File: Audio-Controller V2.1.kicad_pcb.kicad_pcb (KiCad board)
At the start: 2 copper layers, 73 x 100 mm, 12 parts

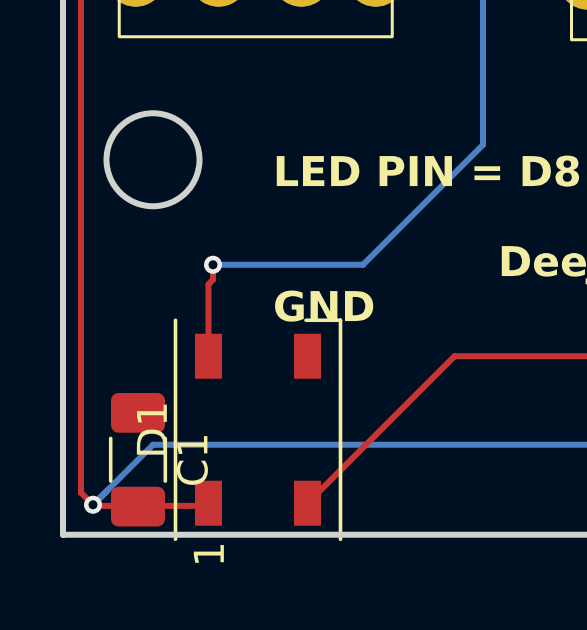
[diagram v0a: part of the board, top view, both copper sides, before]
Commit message: small corrections
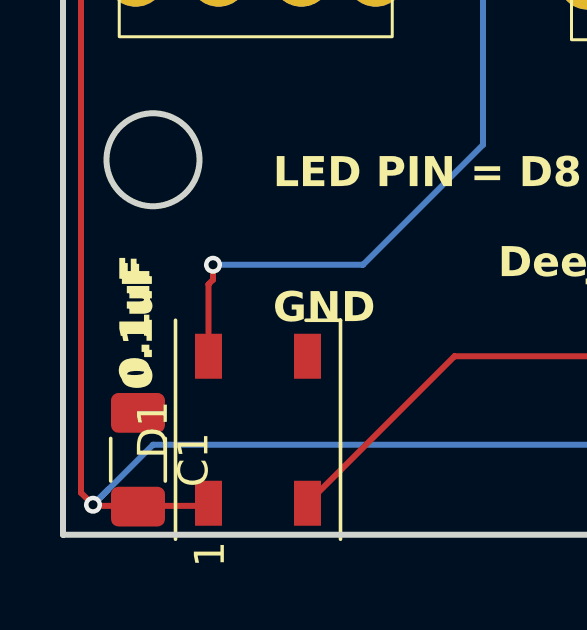
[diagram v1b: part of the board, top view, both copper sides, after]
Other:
- board text added: "0.1uF"
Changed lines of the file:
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@@
 		)
 		(property "Value" "0.1uF"
-			(at 0 1.85 90)
-			(layer "F.Fab")
-			(effects
-				(font
-					(size 1 1)
-					(thickness 0.15)
+			(at -4.5 0 90)
+			(layer "F.SilkS")
+			(effects
+				(font
+					(size 1 1)
+					(thickness 0.2)
+					(bold yes)
 				)
 			)
@@
 		(layer "F.SilkS")
 		(effects
+			(font
+				(size 1 1)
+				(thickness 0.2)
+				(bold yes)
+			)
+			(justify left bottom)
+		)
+	)
+	(gr_text "0.1uF"
+		(at 51 111.5 90)
+		(layer "F.SilkS")
+		(effects
